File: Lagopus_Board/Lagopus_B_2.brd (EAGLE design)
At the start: 20.3 x 58.4 mm, 10 parts, among them J1 PTH, U1 SHT31-DIS-F, U3 BME280, U4 TMP117

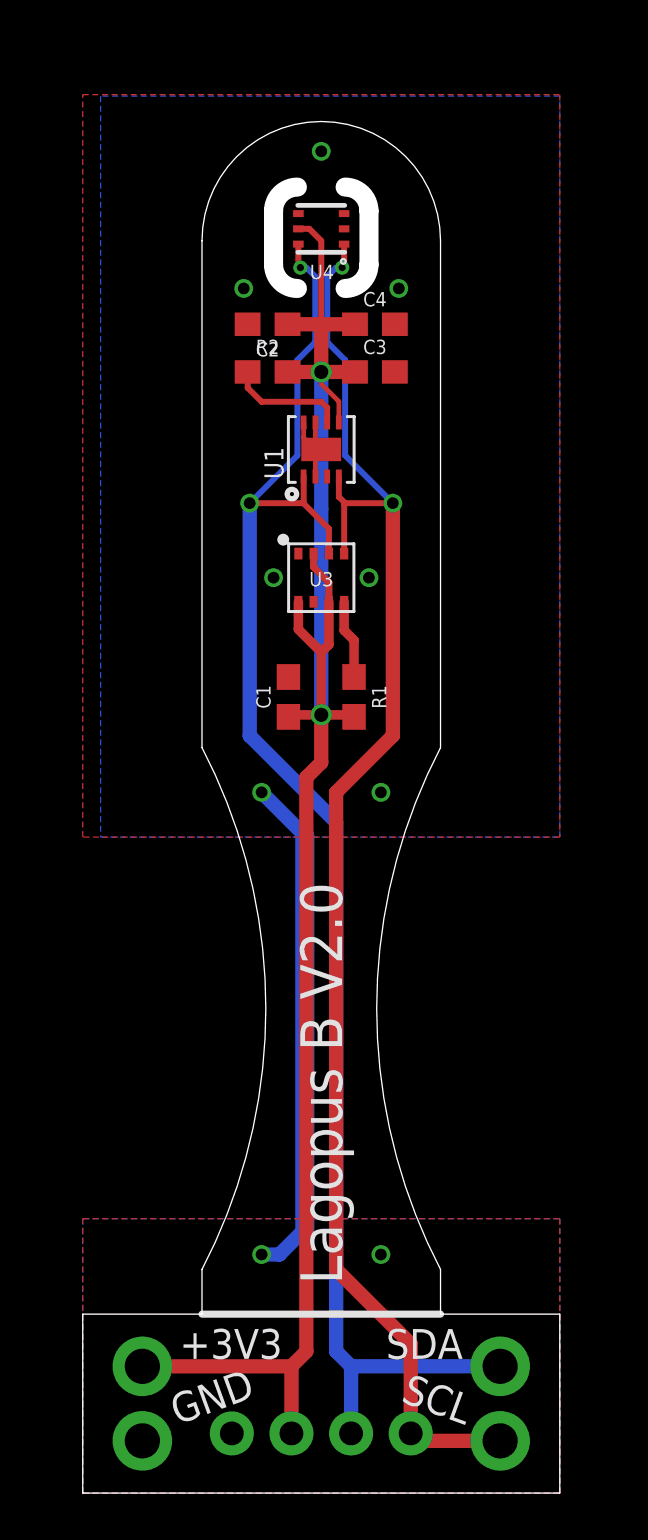
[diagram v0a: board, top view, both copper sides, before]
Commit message: WSN 2 ready for quotations
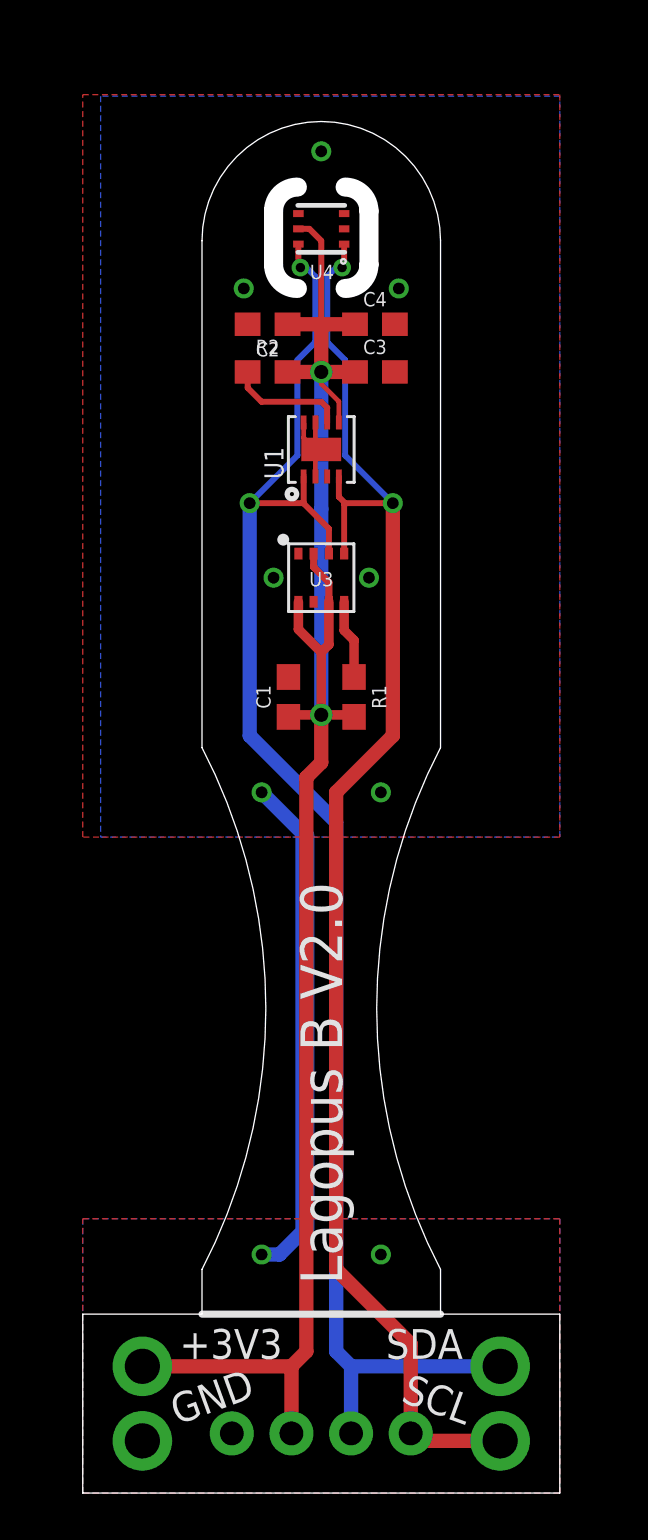
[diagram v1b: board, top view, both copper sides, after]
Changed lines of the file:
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@@
 </class>
 </classes>
-<designrules name="dirt_cheap_dirty_boards.v1">
-<description language="en">&lt;b&gt;Dirty Cheap Dirty Board Design Rules&lt;/b&gt;
-&lt;br&gt;
-&lt;br&gt;Min width/Spacing: 5/5mil
-&lt;br&gt;Min diameter of finished hole 12mil</description>
+<designrules name="SparkFun-2-layer-TIGHT">
+<description language="en">&lt;b&gt;SparkFun 2 Layer Design Rule Checks - STANDARD/TIGHT/FAB-LIMIT&lt;/b&gt;
+&lt;p&gt;
+These rules have been curated by SparkFuns DFM commitee. After doing much research, communicating with our multiple fab houses, and getting quotes of various designs, we have compiled three DRU files.
+&lt;p&gt;
+&lt;b&gt;STANDARD:&lt;/b&gt; This is more of a &quot;best case scenario&quot; set of limitations. If your design has the space, and/or you have the time to work within these parameters, please do. Larger trace width and clearance makes for easier visual inspection of the PCB while troubleshooting (useful in production and to the end user). It also allows for better ability to hack a trace (if you are crazy enough to scrape away the mask and solder to a trace). Another thing to keep in mind is that more metal is just more robust.
+&lt;p&gt;
+&lt;b&gt;TIGHT:&lt;/b&gt; This is where cost comes into play. We have found that most fab houses begin to add extra charges when you go smaller than these specs. In some cases, going to less than 15 mil trace can increase the cost by 10%. (This is why we have set the min drill on this DRU to 15 mil) Same story for traces thinner than 7 mil. To avoid those extra charges, then stay within the rules of this DRU.
+&lt;p&gt;
+&lt;b&gt;FAB-LIMIT:&lt;/b&gt; These set of rules are at the very limit of most fab houses capabilities. You will pay more for these specs, and it should be used on designs that have a darned good reason to need 4 mil vias and 4 mil traces.
+&lt;p&gt;
+**NOTE Clearance, Distance, Sizes, and Restring are all set to different limits in each of these three DRU files. Please compare the files within the CAM job editor window of eagle to see all the numbers.
+&lt;p&gt;
+***NOTE, Please set your Net Classes to default (0mil for all settings), so that it won't effect the DRC when you run it with these settings.</description>
 <param name="layerSetup" value="(1*16)"/>
-<param name="mtCopper" value="0.035mm 0.0175mm 0.035mm 0.035mm 0.035mm 0.035mm 0.035mm 0.035mm 0.035mm 0.035mm 0.035mm 0.035mm 0.035mm 0.035mm 0.0175mm 0.035mm"/>
-<param name="mtIsolate" value="1.5mm 1.1mm 0.2mm 0.15mm 0.2mm 0.15mm 0.2mm 0.15mm 0.2mm 0.15mm 0.2mm 0.15mm 0.2mm 0.15mm 0.2mm"/>
-<param name="mdWireWire" value="5mil"/>
-<param name="mdWirePad" value="5mil"/>
-<param name="mdWireVia" value="5mil"/>
-<param name="mdPadPad" value="5mil"/>
-<param name="mdPadVia" value="5mil"/>
-<param name="mdViaVia" value="5mil"/>
-<param name="mdSmdPad" value="0mil"/>
-<param name="mdSmdVia" value="0mil"/>
-<param name="mdSmdSmd" value="0mil"/>
+<param name="mtCopper" value="0.035mm 0.035mm 0.035mm 0.035mm 0.035mm 0.035mm 0.035mm 0.035mm 0.035mm 0.035mm 0.035mm 0.035mm 0.035mm 0.035mm 0.035mm 0.035mm"/>
+<param name="mtIsolate" value="1.5mm 0.15mm 0.2mm 0.15mm 0.2mm 0.15mm 0.2mm 0.15mm 0.2mm 0.15mm 0.2mm 0.15mm 0.2mm 0.15mm 0.2mm"/>
+<param name="mdWireWire" value="7mil"/>
+<param name="mdWirePad" value="7mil"/>
+<param name="mdWireVia" value="7mil"/>
+<param name="mdPadPad" value="7mil"/>
+<param name="mdPadVia" value="7mil"/>
+<param name="mdViaVia" value="7mil"/>
+<param name="mdSmdPad" value="7mil"/>
+<param name="mdSmdVia" value="7mil"/>
+<param name="mdSmdSmd" value="7mil"/>
 <param name="mdViaViaSameLayer" value="8mil"/>
 <param name="mnLayersViaInSmd" value="2"/>
-<param name="mdCopperDimension" value="10mil"/>
-<param name="mdDrill" value="10mil"/>
+<param name="mdCopperDimension" value="7mil"/>
+<param name="mdDrill" value="7mil"/>
 <param name="mdSmdStop" value="0mil"/>
-<param name="msWidth" value="5mil"/>
-<param name="msDrill" value="12mil"/>
-<param name="msMicroVia" value="12mil"/>
+<param name="msWidth" value="7mil"/>
+<param name="msDrill" value="15mil"/>
+<param name="msMicroVia" value="9.99mm"/>
 <param name="msBlindViaRatio" value="0.5"/>
 <param name="rvPadTop" value="0.25"/>
@@
 <param name="rvMicroViaOuter" value="0.25"/>
 <param name="rvMicroViaInner" value="0.25"/>
-<param name="rlMinPadTop" value="10mil"/>
+<param name="rlMinPadTop" value="7mil"/>
 <param name="rlMaxPadTop" value="20mil"/>
-<param name="rlMinPadInner" value="10mil"/>
+<param name="rlMinPadInner" value="7mil"/>
 <param name="rlMaxPadInner" value="20mil"/>
-<param name="rlMinPadBottom" value="10mil"/>
+<param name="rlMinPadBottom" value="7mil"/>
 <param name="rlMaxPadBottom" value="20mil"/>
-<param name="rlMinViaOuter" value="6mil"/>
+<param name="rlMinViaOuter" value="7mil"/>
 <param name="rlMaxViaOuter" value="20mil"/>
-<param name="rlMinViaInner" value="6mil"/>
+<param name="rlMinViaInner" value="7mil"/>
 <param name="rlMaxViaInner" value="20mil"/>
 <param name="rlMinMicroViaOuter" value="4mil"/>
@@
 <param name="psTop" value="-1"/>
 <param name="psBottom" value="-1"/>
-<param name="psFirst" value="0"/>
+<param name="psFirst" value="-1"/>
 <param name="psElongationLong" value="100"/>
 <param name="psElongationOffset" value="100"/>
 <param name="mvStopFrame" value="1"/>
 <param name="mvCreamFrame" value="0"/>
-<param name="mlMinStopFrame" value="2mil"/>
-<param name="mlMaxStopFrame" value="2mil"/>
+<param name="mlMinStopFrame" value="4mil"/>
+<param name="mlMaxStopFrame" value="4mil"/>
 <param name="mlMinCreamFrame" value="0mil"/>
 <param name="mlMaxCreamFrame" value="0mil"/>
@@
 <param name="checkAngle" value="0"/>
 <param name="checkFont" value="1"/>
-<param name="checkRestrict" value="0"/>
+<param name="checkRestrict" value="1"/>
 <param name="checkStop" value="0"/>
 <param name="checkValues" value="0"/>
@@
 <contactref element="U4" pad="1"/>
 <contactref element="U1" pad="4"/>
-<via x="0.889" y="44.577" extent="1-16" drill="0.3048"/>
+<via x="0.889" y="44.577" extent="1-16" drill="0.4"/>
 <via x="3.048" y="34.544" extent="1-16" drill="0.5"/>
 <wire x1="3.048" y1="34.544" x2="1.016" y2="34.544" width="0.254" layer="1"/>
@@
 <contactref element="U4" pad="6"/>
 <contactref element="U1" pad="1"/>
-<via x="-0.889" y="44.577" extent="1-16" drill="0.3048"/>
+<via x="-0.889" y="44.577" extent="1-16" drill="0.4"/>
 <via x="-3.048" y="34.544" extent="1-16" drill="0.5"/>
 <wire x1="-3.048" y1="34.544" x2="-0.762" y2="34.544" width="0.254" layer="1"/>

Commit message: Order of v2
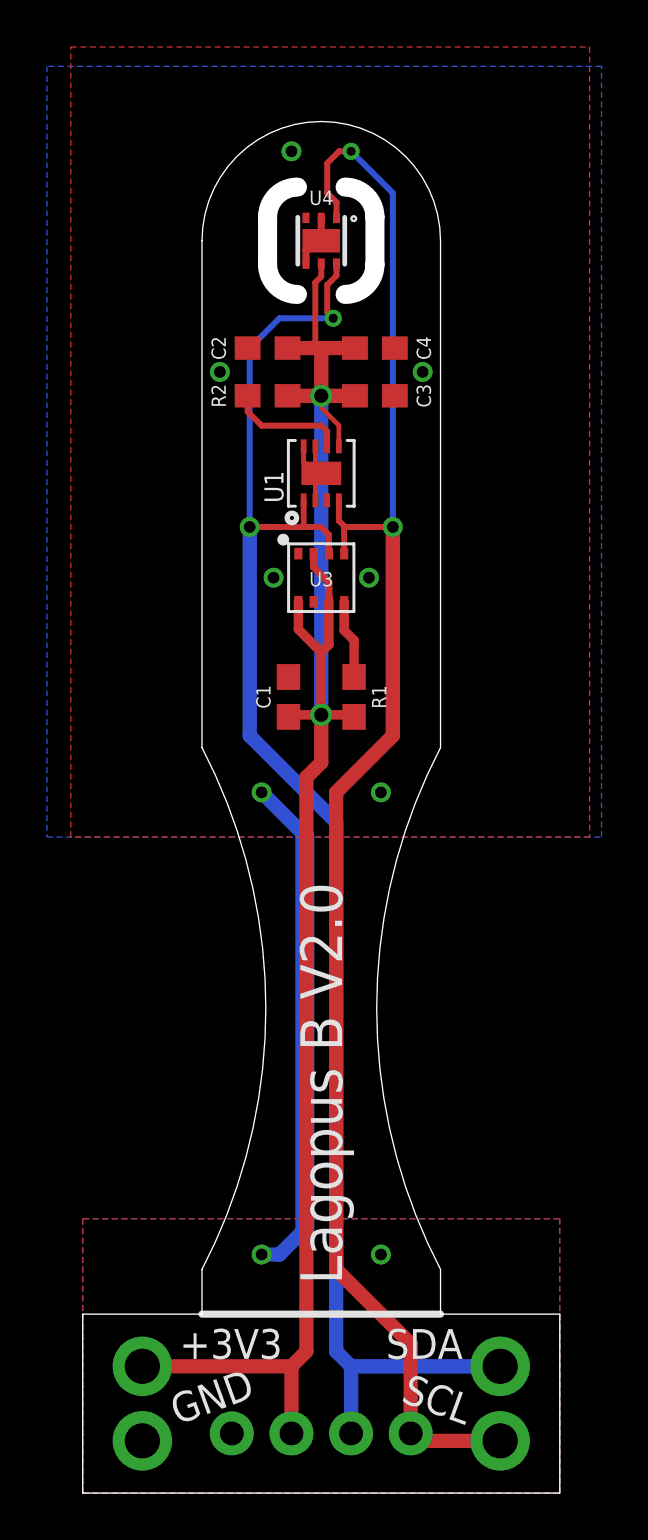
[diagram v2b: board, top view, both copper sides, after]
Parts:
- U1: device microbuilder:SHT3X -> Lagopus_B_2:SHT3X
- U4: device SparkFun-Sensors:TMP117 -> Lagopus_B_2:TMP117
- moved C2 1.02 mm to (-2.29, 41.1)
- moved C3 1.02 mm to (2.29, 39.1)
- moved C4 1.02 mm to (2.29, 41.1)
- moved R2 1.02 mm to (-2.29, 39.1)
- moved U1 1.02 mm to (0.00, 35.8)
- moved U4 0.51 mm to (0.00, 45.7), turned to 270 degrees
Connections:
- net GND: now also U4.THERMAL
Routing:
- net SCL: track 64.0 -> 69.8 mm
- net GND: track 25.7 -> 28.1 mm
- net 3.3V: track 79.8 -> 77.8 mm
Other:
- outline, holes or cut-outs redrawn
